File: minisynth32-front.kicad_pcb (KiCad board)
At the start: 2 copper layers, 15.2 x 89.9 mm, 5 parts, among them J6 R_BREAKOUT, J7 SSD1306 OLED, SW1 B1, SW3 B2

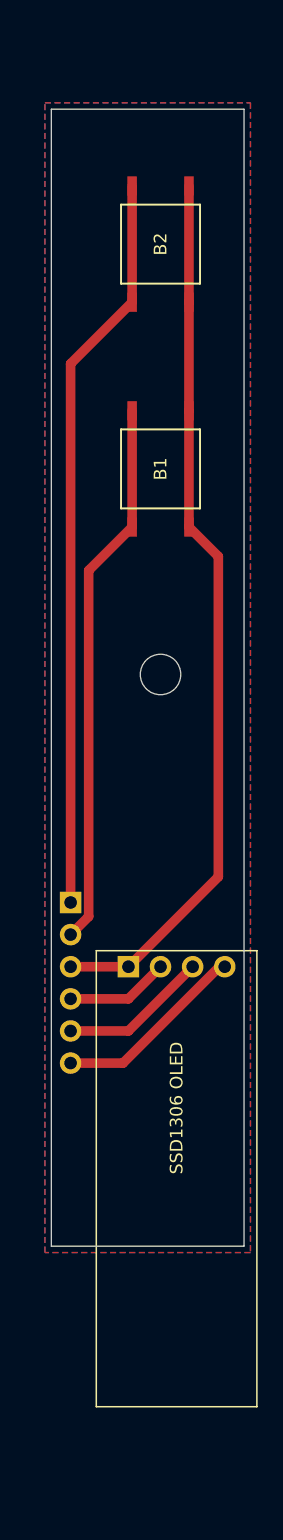
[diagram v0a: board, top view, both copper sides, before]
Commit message: front pcb v2
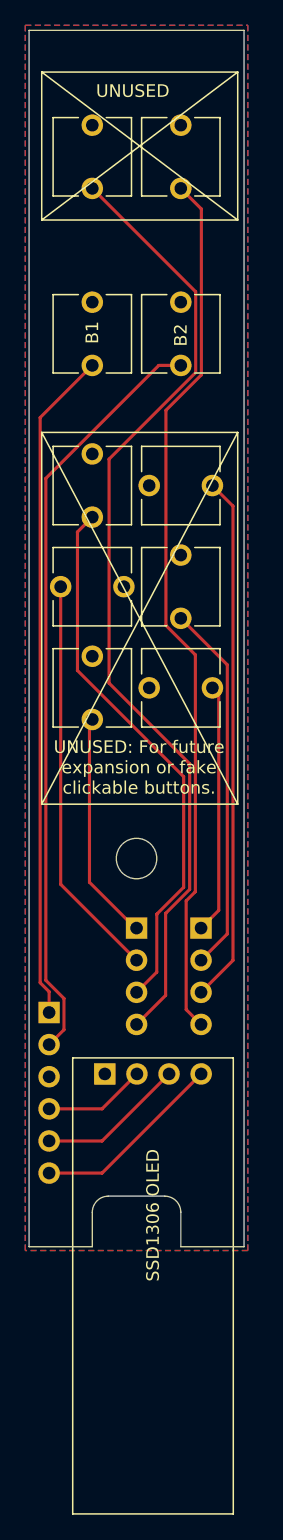
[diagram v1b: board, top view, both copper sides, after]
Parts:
- added J8: UNUSED_2, minisynth32:PinHeader_1x04_P2.54mm_Vertical, B.Cu at (123.6, 114.8)
- added J9: UNUSED_1, minisynth32:PinHeader_1x04_P2.54mm_Vertical, B.Cu at (118.5, 114.8)
- added SW10: SW_Push, minisynth32:TL59N, F.Cu at (122.0, 79.8)
- added SW2: B2, minisynth32:TL59N, F.Cu at (122.0, 67.8)
- added SW4: SW_Push, minisynth32:TL59N, F.Cu at (122.0, 53.8)
- added SW5: SW_Push, minisynth32:TL59N, F.Cu at (115.0, 95.8)
- added SW6: SW_Push, minisynth32:TL59N, F.Cu at (115.0, 87.8)
- added SW7: SW_Push, minisynth32:TL59N, F.Cu at (115.0, 79.8)
- added SW8: SW_Push, minisynth32:TL59N, F.Cu at (122.0, 95.8)
- added SW9: SW_Push, minisynth32:TL59N, F.Cu at (122.0, 87.8)
- SW1: footprint minisynth32:TL3301AF160QG-nopaste -> minisynth32:TL59N
- SW3: value B2 -> SW_Push; footprint minisynth32:TL3301AF160QG-nopaste -> minisynth32:TL59N
- moved REF** 14.7 mm to (118.5, 109.3)
- moved SW1 12.0 mm to (115.0, 67.8), turned to 0 degrees
- moved J6 8.86 mm to (111.6, 121.5)
- moved SW3 8.76 mm to (115.0, 53.8), turned to 0 degrees
- moved J7 8.68 mm to (119.8, 143.1)
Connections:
- J6 pad 3: Net-(J6-Pad3) -> GND2
- J7 pad 1: Net-(J6-Pad3) -> GND2
- SW1 pad 1: Net-(J6-Pad3) -> Net-(J6-Pad1)
- SW1 pad 2: Net-(J6-Pad3) -> GND2
- SW3 pad 1: Net-(J6-Pad3) -> Net-(J9-Pad4)
- SW3 pad 2: Net-(J6-Pad3) -> GND2
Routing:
- net Net-(J9-Pad4): track 0.00 -> 76.7 mm
- net Net-(J6-Pad3): track 70.2 -> 0.00 mm
- net Net-(J8-Pad4): track 0.00 -> 69.7 mm
- net Net-(J9-Pad3): track 0.00 -> 43.1 mm
- net Net-(J8-Pad3): track 0.00 -> 41.8 mm
- net Net-(J9-Pad2): track 0.00 -> 32.0 mm
- net Net-(J8-Pad2): track 0.00 -> 29.4 mm
- net Net-(J8-Pad1): track 0.00 -> 19.8 mm
- net Net-(J9-Pad1): track 0.00 -> 18.2 mm
- net Net-(J6-Pad2): track 43.4 -> 60.2 mm
- net Net-(J6-Pad1): track 58.7 -> 53.2 mm
- added copper zone on B.Cu, net GND2
- removed copper zone on B.Cu, net (none)
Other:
- board size 15.2 x 89.9 mm -> 17 x 96.2 mm
- board text added: "B2 B1"
- board text added: "Minisynth 32: Front panel board Rev 2.0 https://github.com/grantek/minisynth32"
- board text added: "UNUSED"
- board text added: "UNUSED: For future expansion or fake clickable buttons."
- board text removed: "B1 B2"
- board text removed: "Minisynth 32: Front panel board https://github.com/grantek/minisynth32 Rev 1.1"
